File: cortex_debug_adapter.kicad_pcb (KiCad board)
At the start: 2 copper layers, 2 parts, among them J1 Conn_02x05_Odd_Even, J2 Conn_01x07_Male

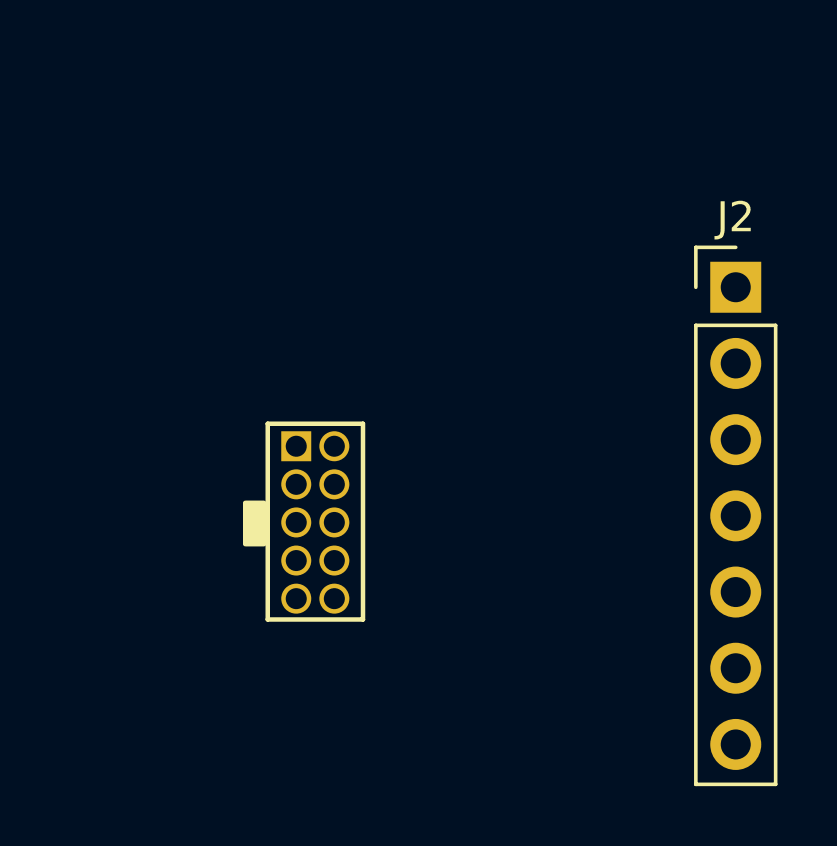
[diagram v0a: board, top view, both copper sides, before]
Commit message: PCB done
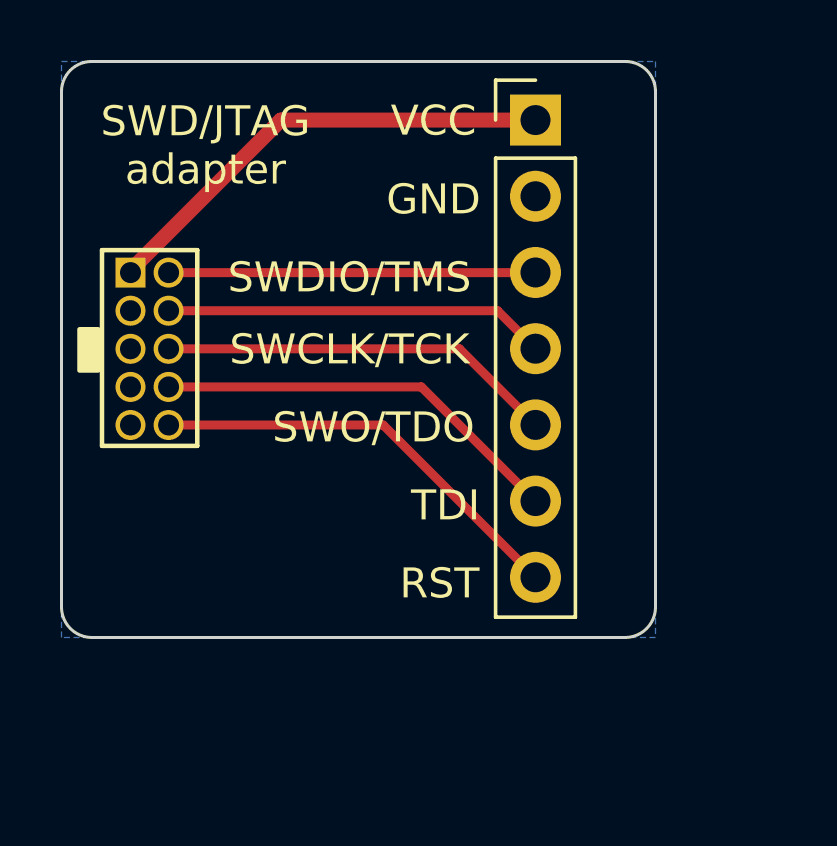
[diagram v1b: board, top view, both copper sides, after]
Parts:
- added kibuzzard-62A19C5B: G***, kibuzzard-62A19C5B, B.Cu at (153.6, 100.6)
- moved J2 8.70 mm to (160.8, 93.0)
- moved J1 8.00 mm to (147.3, 98.0)
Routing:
- net VCC: track 0.00 -> 15.6 mm
- net /RESET: track 0.00 -> 14.3 mm
- net /TDI: track 0.00 -> 13.8 mm
- net /TDO/SWO: track 0.00 -> 13.3 mm
- net /TCLK/SWCLK: track 0.00 -> 12.8 mm
- net /TMS/SWDIO: track 0.00 -> 12.2 mm
- added copper zone on B.Cu, net GND
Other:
- board outline added: 19.8 x 19.2 mm
- board text added: "Designed by"
- board text added: "GND"
- board text added: "RST"
- board text added: "SWCLK/TCK"
- board text added: "SWD/JTAG adapter"
- board text added: "SWDIO/TMS"
- board text added: "SWO/TDO"
- board text added: "TDI"
- board text added: "VCC"
